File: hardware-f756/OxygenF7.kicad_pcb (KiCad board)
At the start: 2 copper layers, 74 x 45 mm, 65 parts, among them J1 Conn_01x04, J10 Micro_SD_Card_Det, J2 USB_C_2.0, J3 JST SH-4, J4 JST ZH-4, J5 Conn_03x08, J6 Conn_01x16, J7 Conn_01x04, J9 1.25mm, SW1 SW_Push, SW2 SW_Push, U1 STM32F756VGTx, U2 XC6220B331MR, U3 MPU-6000, U4 BMP388, U5 W25Q128JVS, Y1 8Mhz

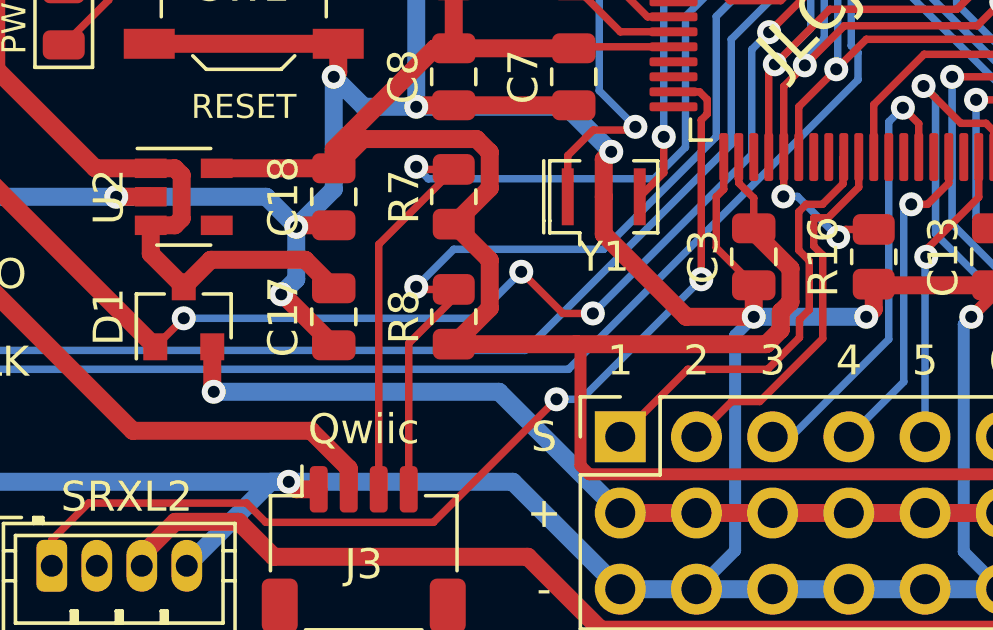
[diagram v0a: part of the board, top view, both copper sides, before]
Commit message: Small tweaks
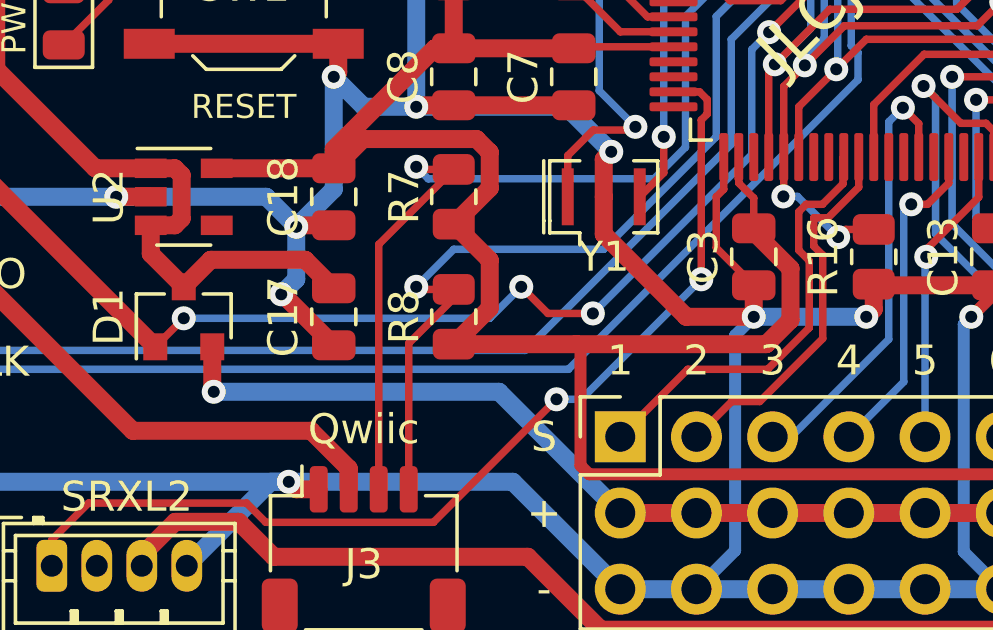
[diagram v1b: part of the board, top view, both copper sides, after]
